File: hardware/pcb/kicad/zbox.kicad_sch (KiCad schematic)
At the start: 16 parts, among them J1 USB_C_Receptacle_USB2.0_14P, J11 PAD_LED_WS2812B, J13 NS4168_SOUND, J2 PAD_BAT_LIPO, J3 PAD_PN532_SPI, J7 PAD_BUTTONS, J8 ESP_LEFT, J9 ESP_RIGHT, Q2 AO3415A, U2 STEPUP_MT3608

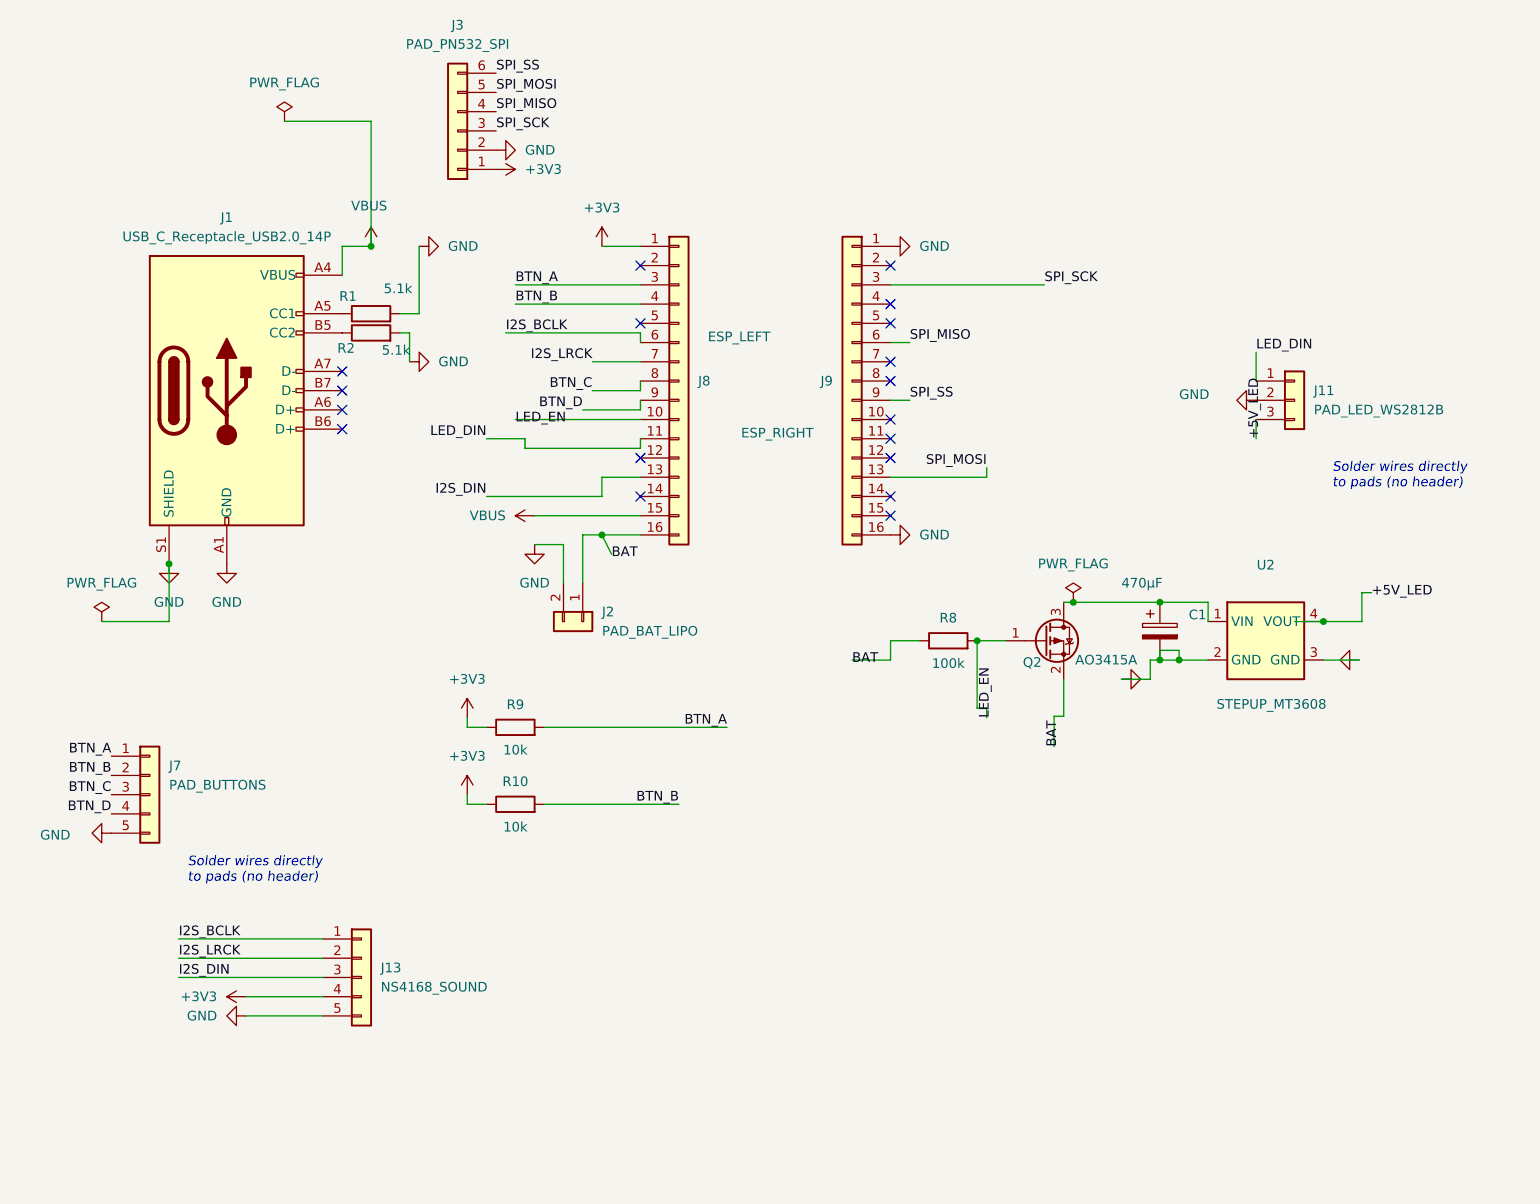
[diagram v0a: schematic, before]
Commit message: documentation update, small fixes
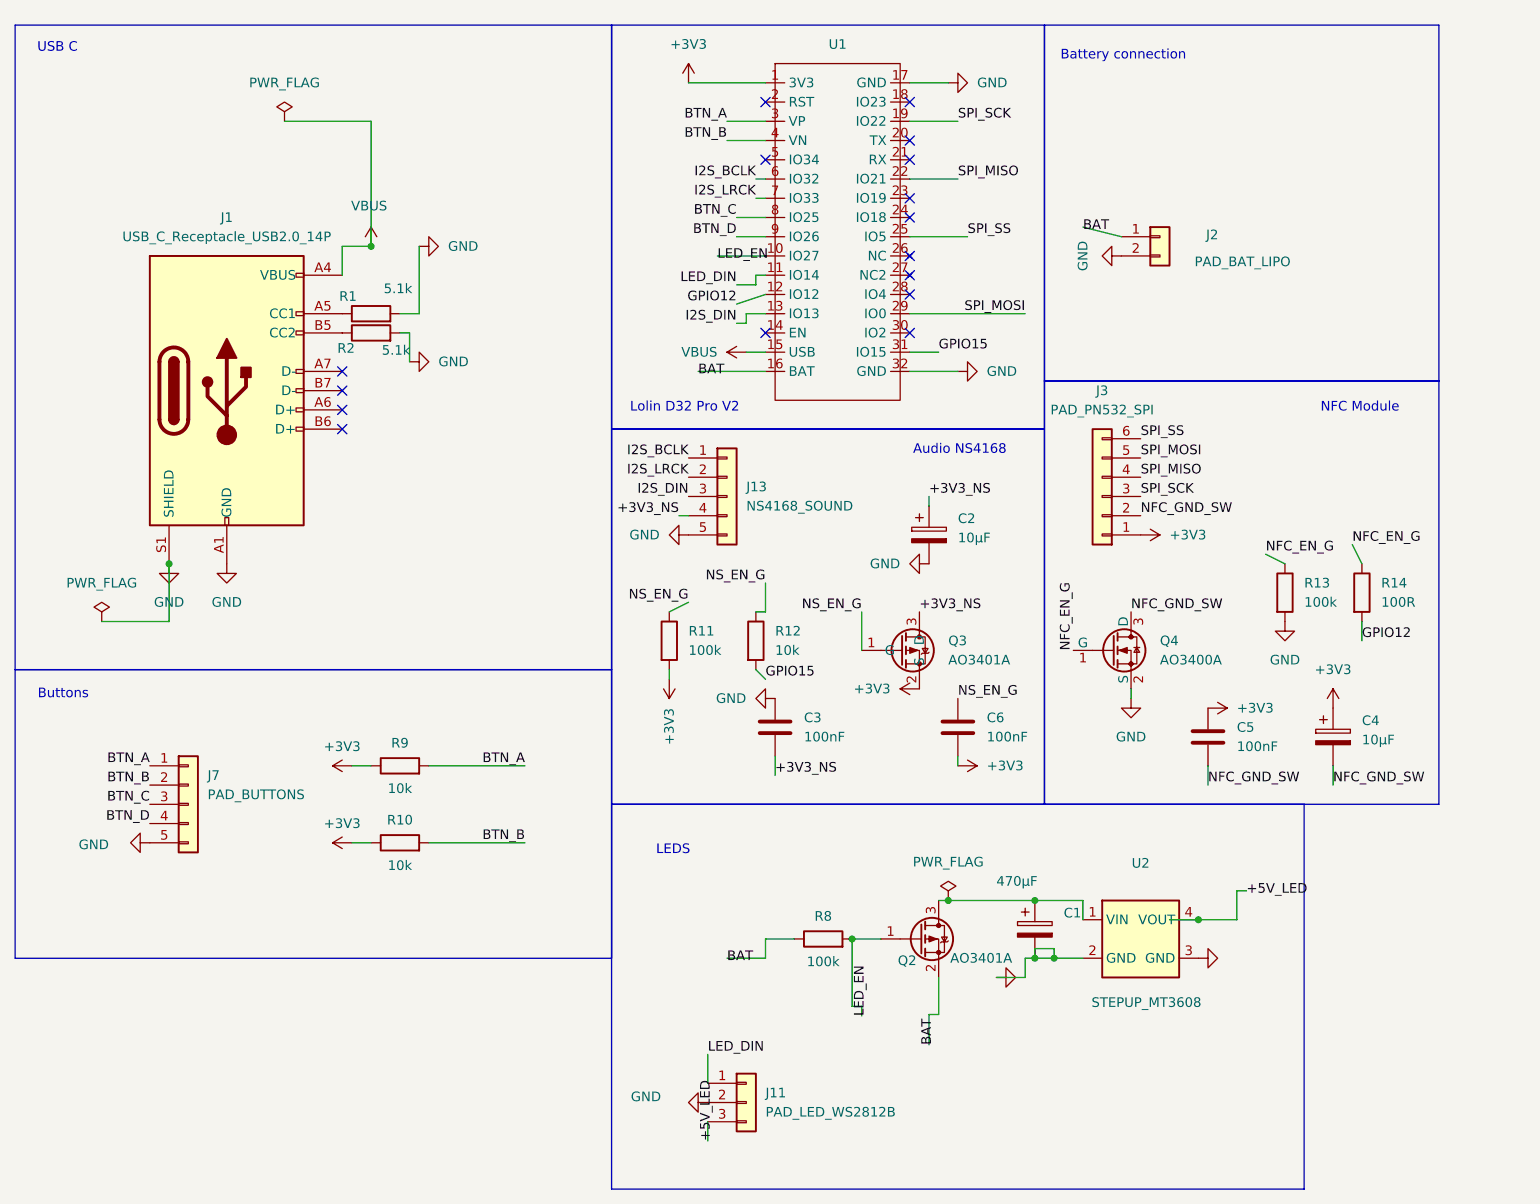
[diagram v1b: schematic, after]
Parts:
- removed J8: ESP_LEFT, Connector_PinHeader_2.54mm:PinHeader_1x16_P2.54mm_Vertical, symbol Connector_Generic:Conn_01x16
- removed J9: ESP_RIGHT, Connector_PinHeader_2.54mm:PinHeader_1x16_P2.54mm_Vertical, symbol Connector_Generic:Conn_01x16
- added C2, C4: 10µF, Capacitor_THT:CP_Radial_D5.0mm_P2.50mm, symbol Device:C_Polarized
- added C3, C5, C6: 100nF, Capacitor_THT:C_Disc_D5.0mm_W2.5mm_P5.00mm, symbol Device:C
- added Q3: AO3401A, Package_TO_SOT_SMD:SOT-23, symbol Transistor_FET:AO3401A
- added Q4: AO3400A, Package_TO_SOT_SMD:SOT-23, symbol Transistor_FET:AO3400A
- added R11, R13: 100k, Resistor_THT:R_Axial_DIN0207_L6.3mm_D2.5mm_P10.16mm_Horizontal, symbol Device:R
- added R12: 10k, Resistor_THT:R_Axial_DIN0207_L6.3mm_D2.5mm_P10.16mm_Horizontal, symbol Device:R
- added R14: 100R, Resistor_THT:R_Axial_DIN0207_L6.3mm_D2.5mm_P10.16mm_Horizontal, symbol Device:R
- added U1: (no value), symbol lolin_hub:Lolin_D32_Pro
- Q2: value AO3415A -> AO3401A
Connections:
- net +3V3: now also C4.1, C5.1, C6.2, Q3.2 (S), R11.2, U1.1 (3V3); no longer J13.4 (Pin_4)
- net BAT: now also U1.16 (BAT)
- net BTN_A: now also U1.3 (VP)
- net BTN_B: now also U1.4 (VN)
- net BTN_C: now also U1.8 (IO25)
- net BTN_D: now also U1.9 (IO26)
- net GND: now also C2.2, C3.1, Q4.2 (S), R13.2, U1.17 (GND), U1.32 (GND); no longer J3.2 (Pin_2)
- net I2S_BCLK: now also U1.6 (IO32)
- net I2S_DIN: now also U1.13 (IO13)
- net I2S_LRCK: now also U1.7 (IO33)
- net LED_DIN: now also U1.11 (IO14)
- net LED_EN: now also U1.10 (IO27)
- net SPI_MISO: now also U1.22 (IO21)
- net SPI_MOSI: now also U1.29 (IO0)
- net SPI_SCK: now also U1.19 (IO22)
- net SPI_SS: now also U1.25 (IO5)
- net VBUS: now also U1.15 (USB)
- new net +3V3_NS: C2.1, C3.2, J13.4 (Pin_4), Q3.3 (D)
- new net GPIO12: R14.2, U1.12 (IO12)
- new net GPIO15: R12.2, U1.31 (IO15)
- new net NFC_EN_G: Q4.1 (G), R13.1, R14.1
- new net NFC_GND_SW: C4.2, C5.2, J3.2 (Pin_2), Q4.3 (D)
- new net NS_EN_G: C6.1, Q3.1 (G), R11.1, R12.1
- no-connect marks 18 -> 16
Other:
- note added: "Audio NS4168"
- note added: "Battery connection"
- note added: "Buttons"
- note added: "LEDS"
- note added: "Lolin D32 Pro V2"
- note added: "NFC Module"
- note added: "USB C"
- note removed: "Solder wires directly to pads (no header)"
- moved on the sheet: C1, J11, J13, J2, J3, J7, Q2, R10, R8, R9, U2
